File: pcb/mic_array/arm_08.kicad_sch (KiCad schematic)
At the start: 16 parts, among them U65 IM72D128V01XTMA1, U66 IM72D128V01XTMA1, U67 IM72D128V01XTMA1, U68 IM72D128V01XTMA1, U69 IM72D128V01XTMA1, U70 IM72D128V01XTMA1, U71 IM72D128V01XTMA1, U72 IM72D128V01XTMA1

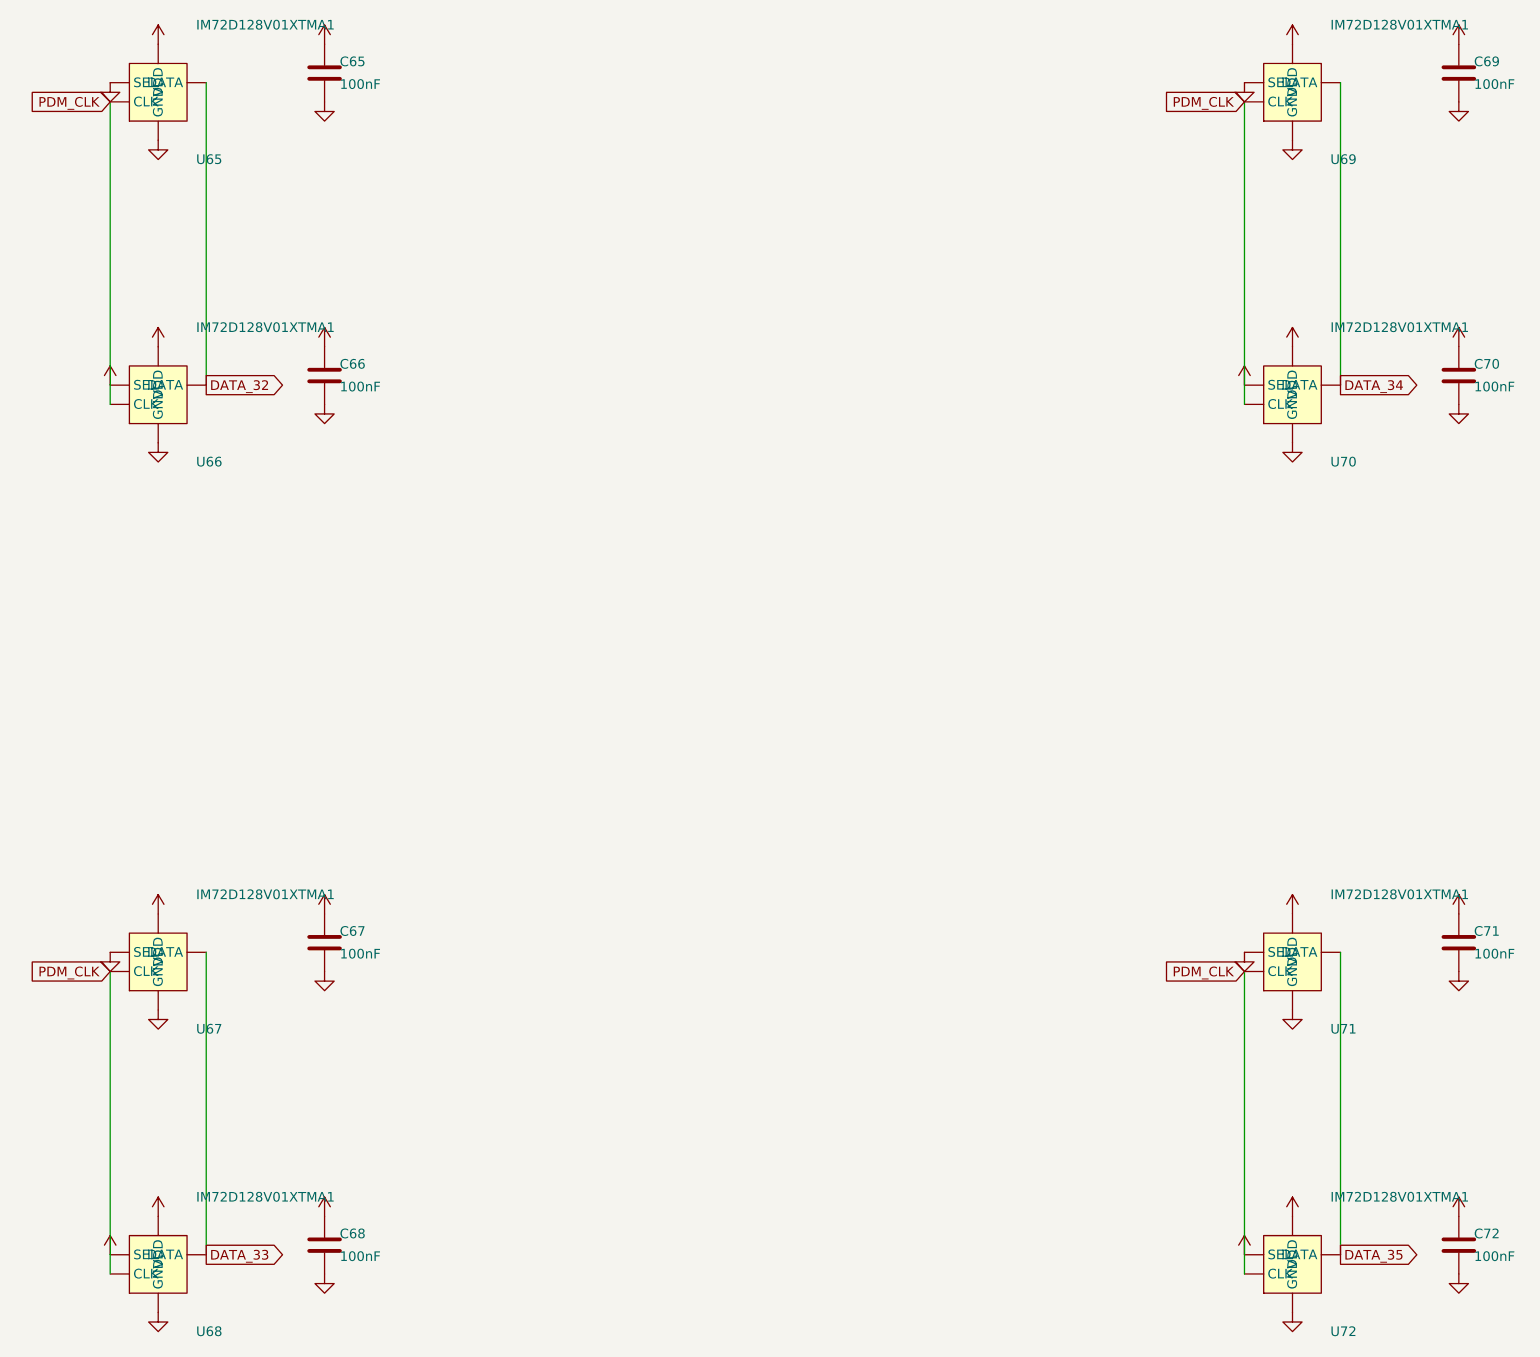
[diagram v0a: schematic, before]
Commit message: Updated.
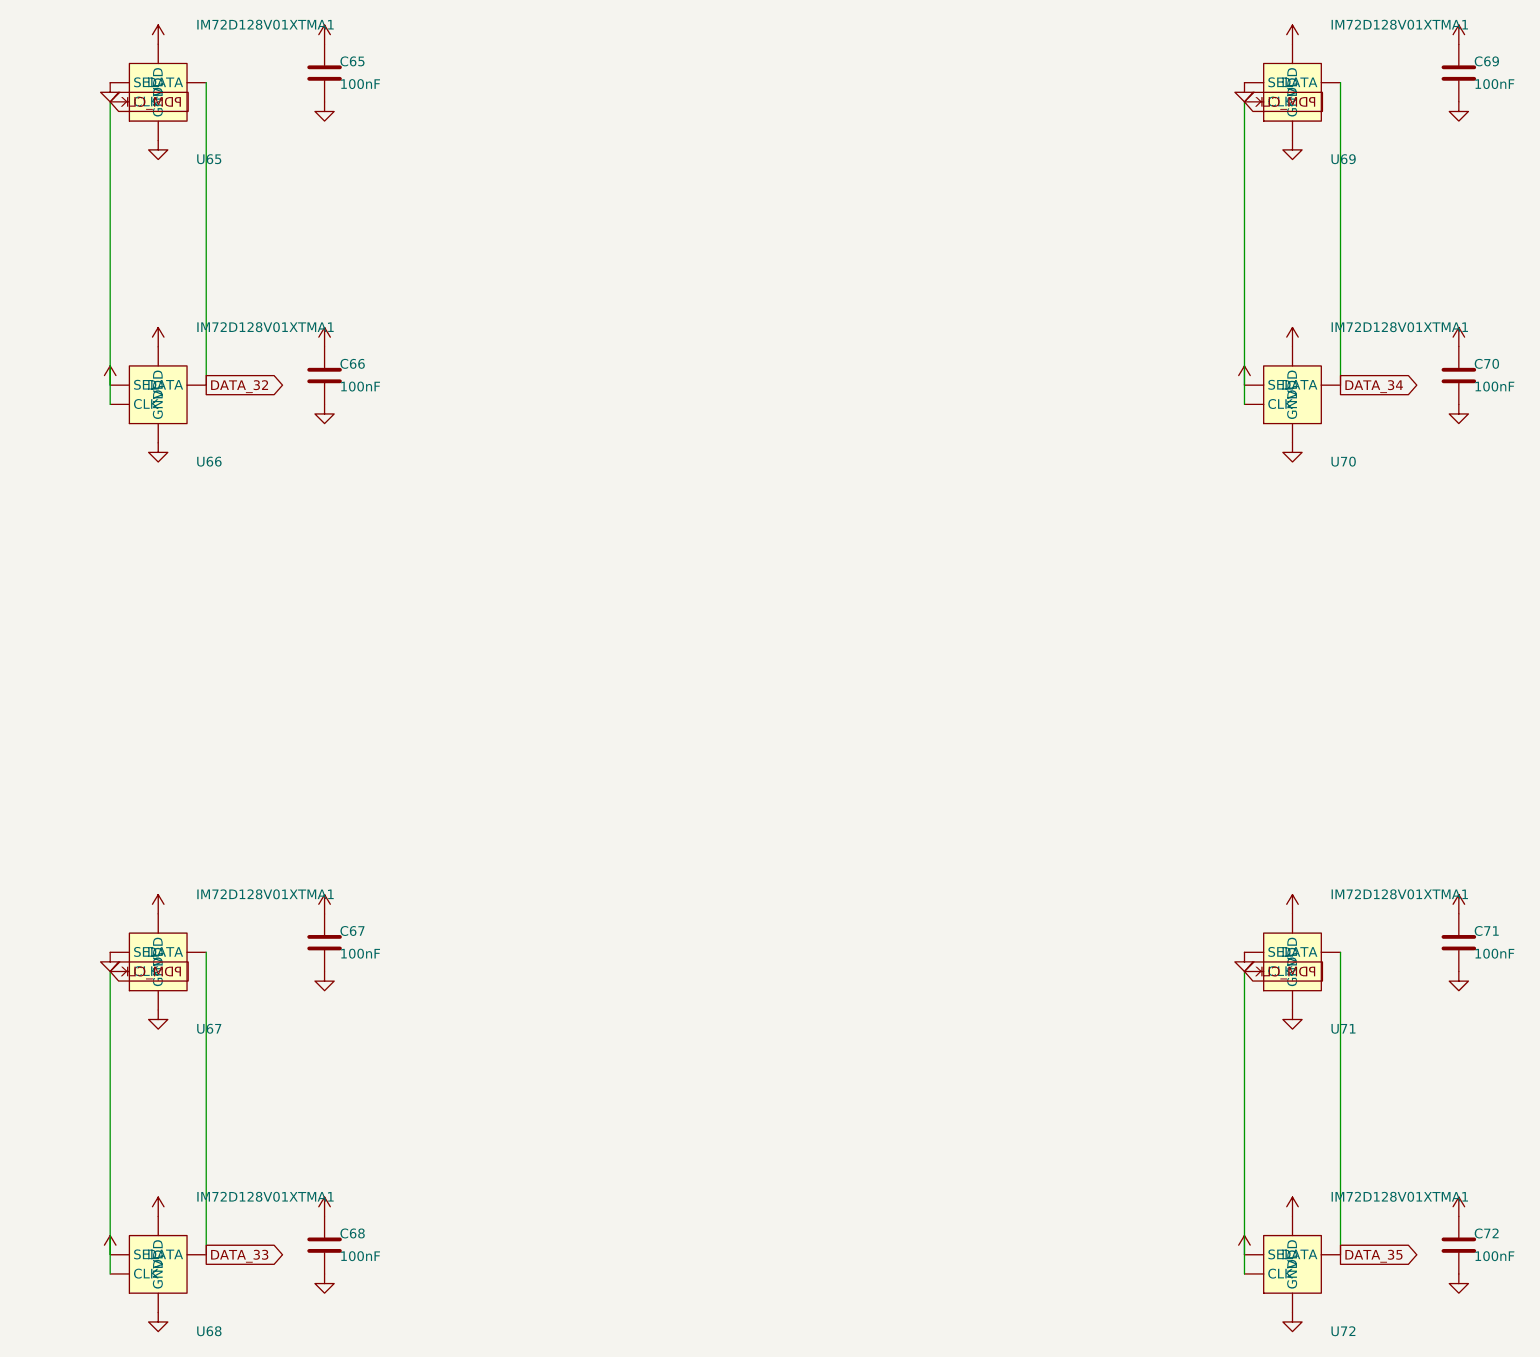
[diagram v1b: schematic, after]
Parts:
- C65, C66, C67, C68, C69, C70, C71, C72: footprint Capacitor_SMD:C_0402_1005Metric -> (none)
- U65, U66, U67, U68, U69, U70, U71, U72: footprint Sensor_Audio:Infineon_PG-LLGA-5-2 -> (none)
